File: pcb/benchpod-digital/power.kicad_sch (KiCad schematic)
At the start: 71 parts, among them J4 DB2ERC-3.81-2P-BK, J5 DB2ERC-3.81-2P-BK, J6 DB2ERC-3.81-2P-BK, U26 TPS259470ARPWR, U27 TPS259470ARPWR, U29 INA226AIDGSR, U30 TPS82130SILR, U31 AP2112K-1.2, U32 AP2112K-2.5TRG1, U33 INA226AIDGSR, U52 AP2112K-1.8TRG1, U56 TCA9554PWR

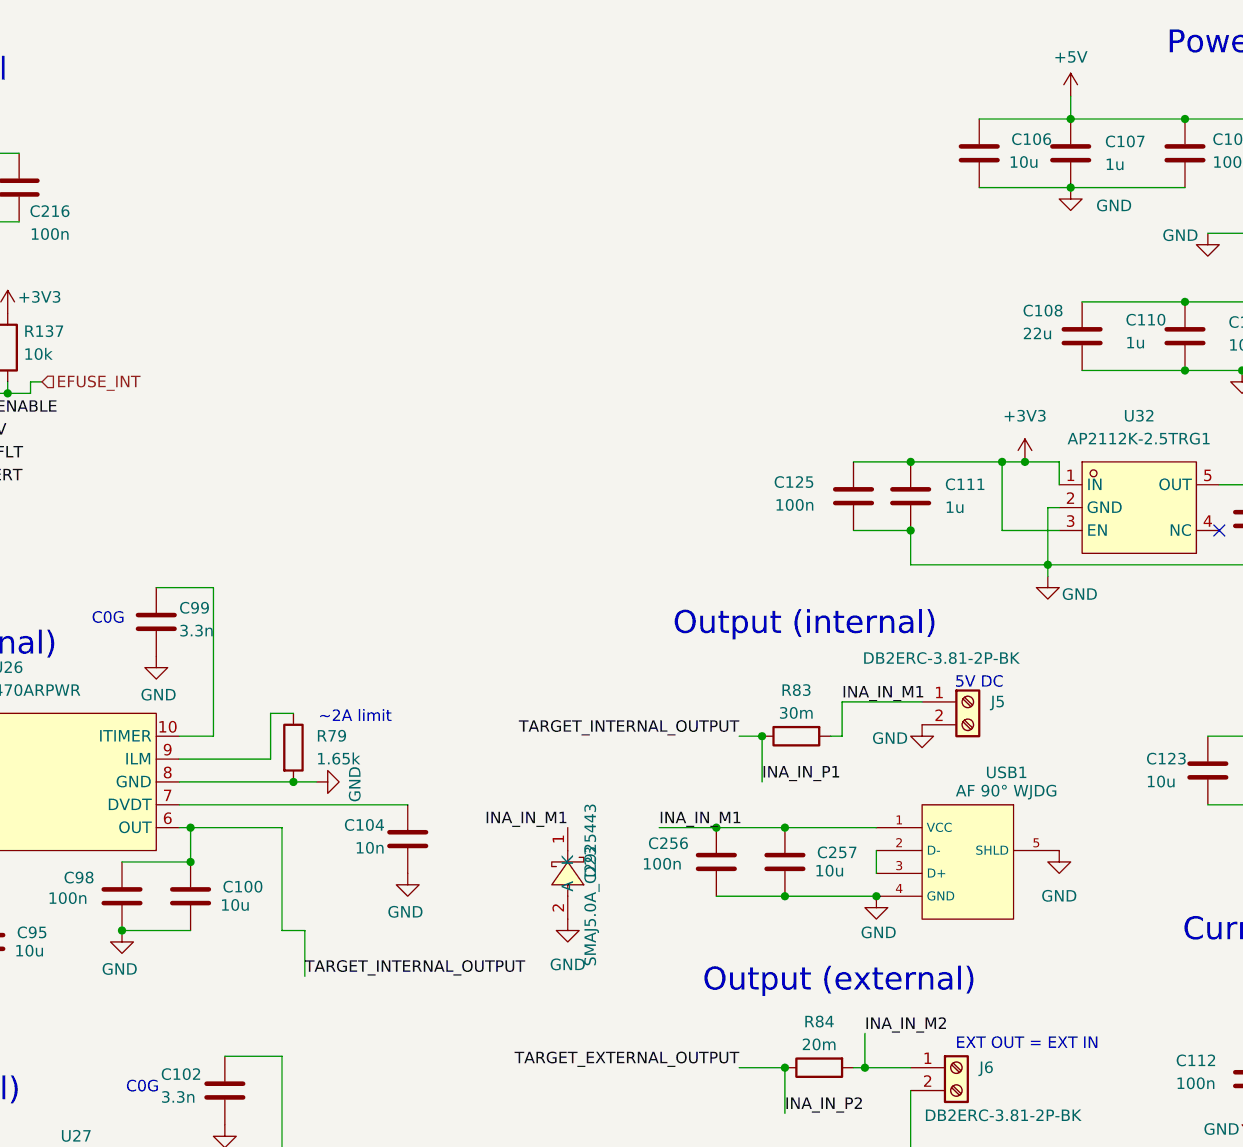
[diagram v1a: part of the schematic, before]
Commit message: pcb work
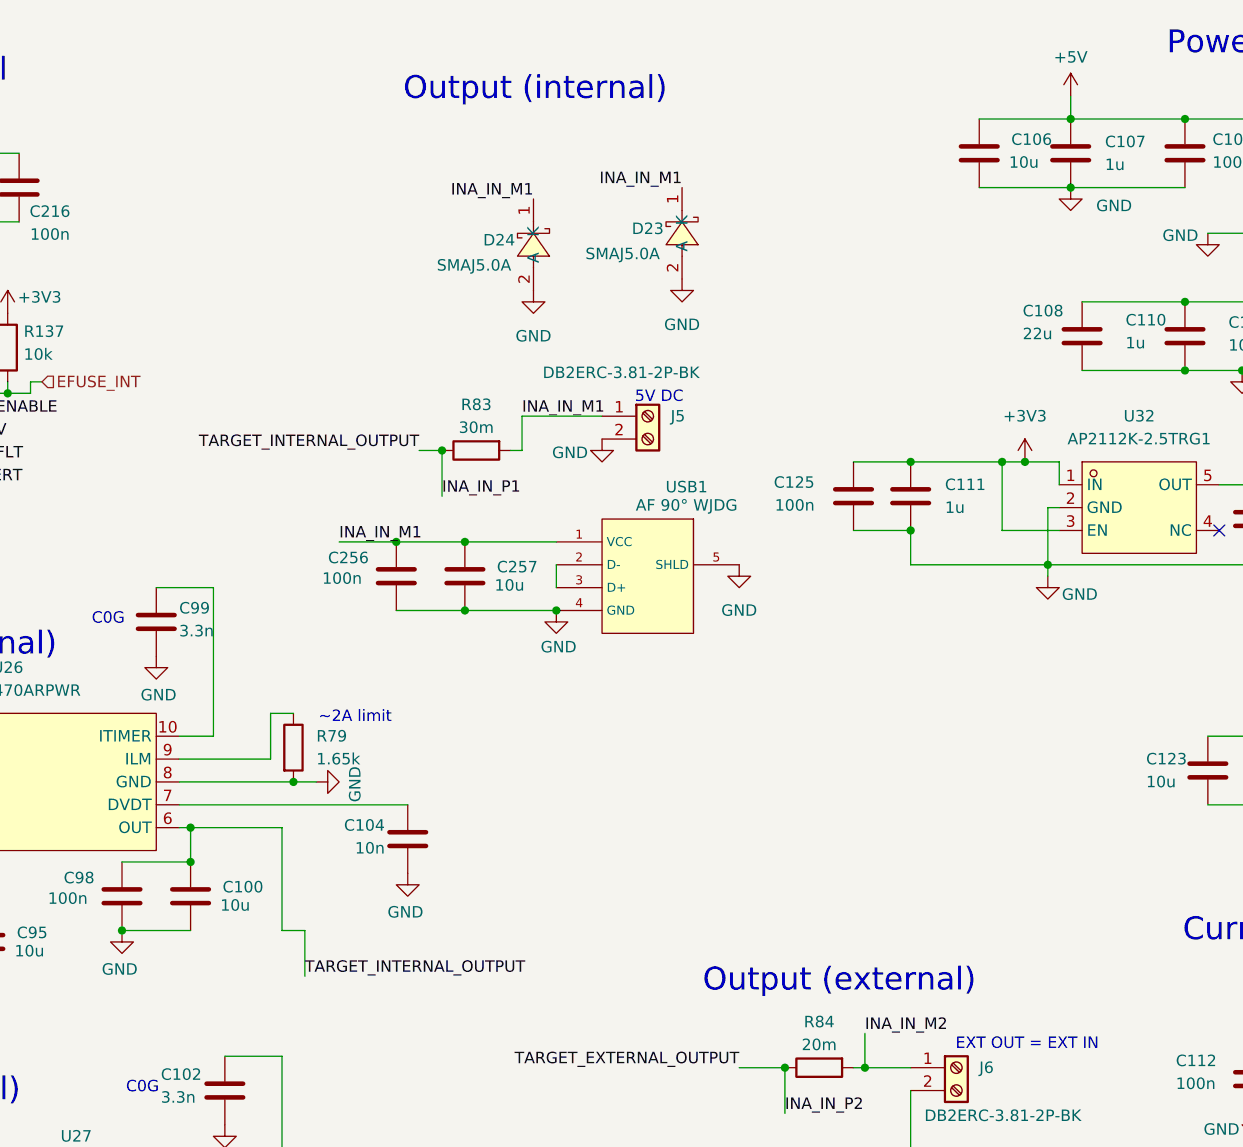
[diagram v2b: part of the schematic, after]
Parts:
- added D24: SMAJ5.0A, lcsc:SMA_L4.3-W2.6-LS5.0-RD, symbol lcsc_lib:SMAJ5.0A_C2925443
- D23: value SMAJ5.0A_C2925443 -> SMAJ5.0A
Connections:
- net GND: now also D24.2 (A)
- net INA_IN_M1: now also D24.1 (K)
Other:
- moved on the sheet: C256, C257, D23, J5, R83, USB1
